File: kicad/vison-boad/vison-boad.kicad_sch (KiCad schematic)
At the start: 29 parts, among them J1 USB_C_Receptacle_USB2.0, J2 Wio Terminal, J3 UART, J4 pin_test, J5 NEO PIXEL, J6 to main, J7 I2C_0, SW1 BOOTSET, SW2 RST, SW3 M1n_RST, U1 RP2040_Stamp, U2 M1n-break, U3 M1n-break, U4 M1n-break, U5 M1n-break, U6 M1n-break

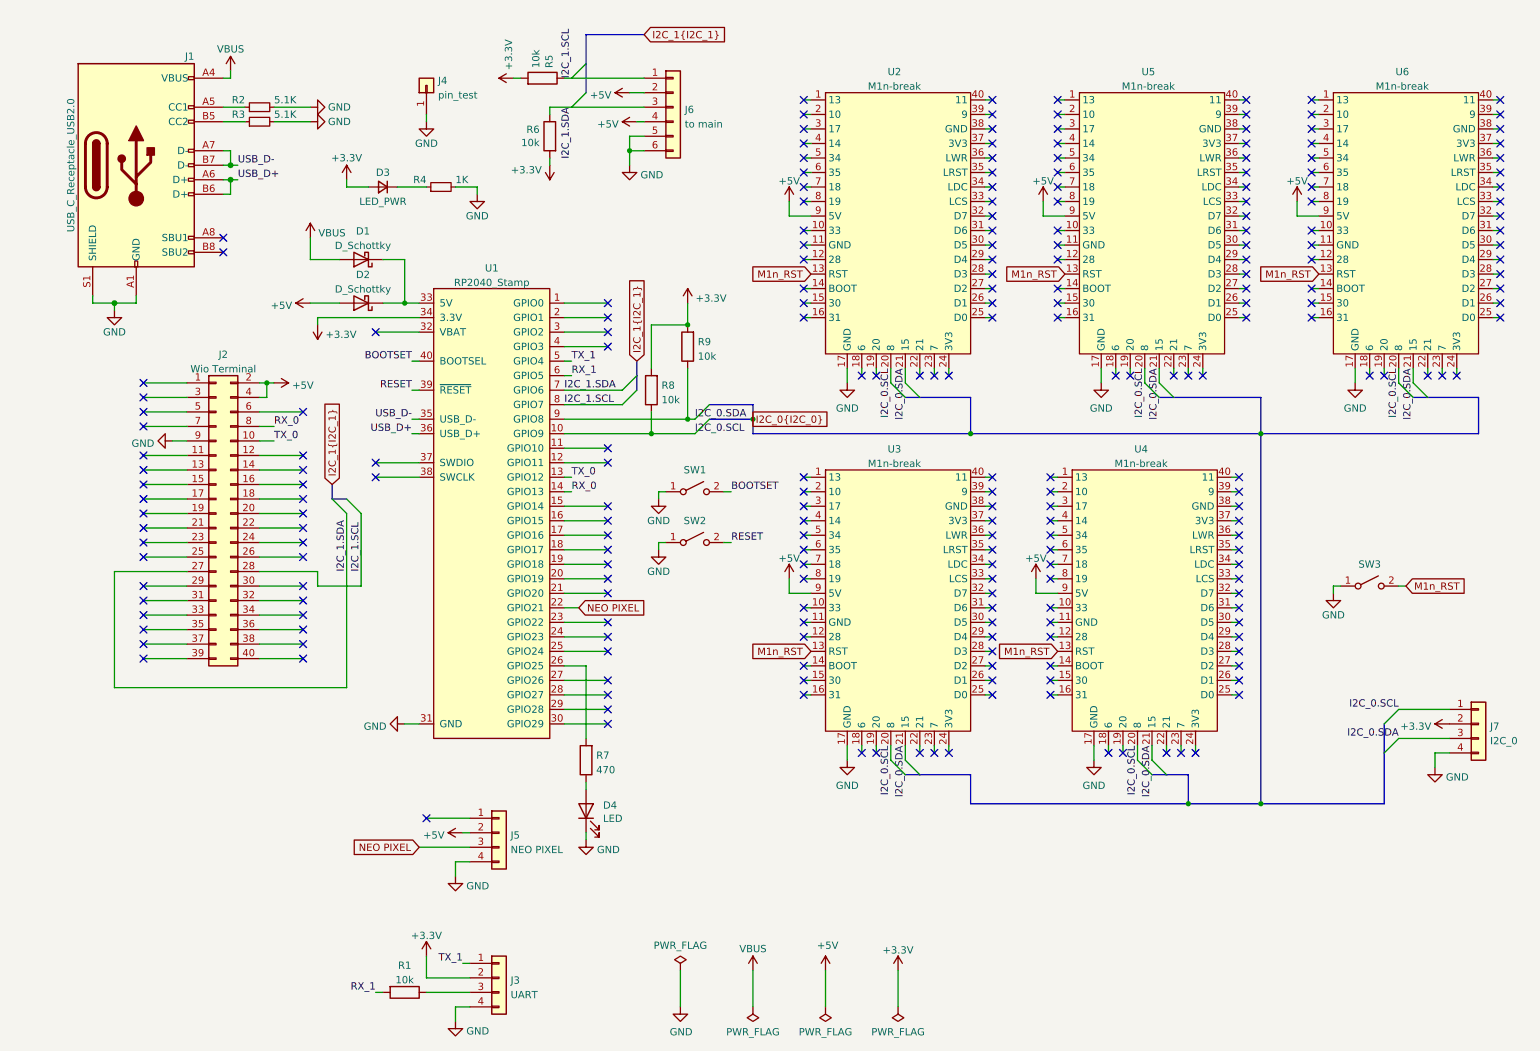
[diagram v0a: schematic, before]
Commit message: bus
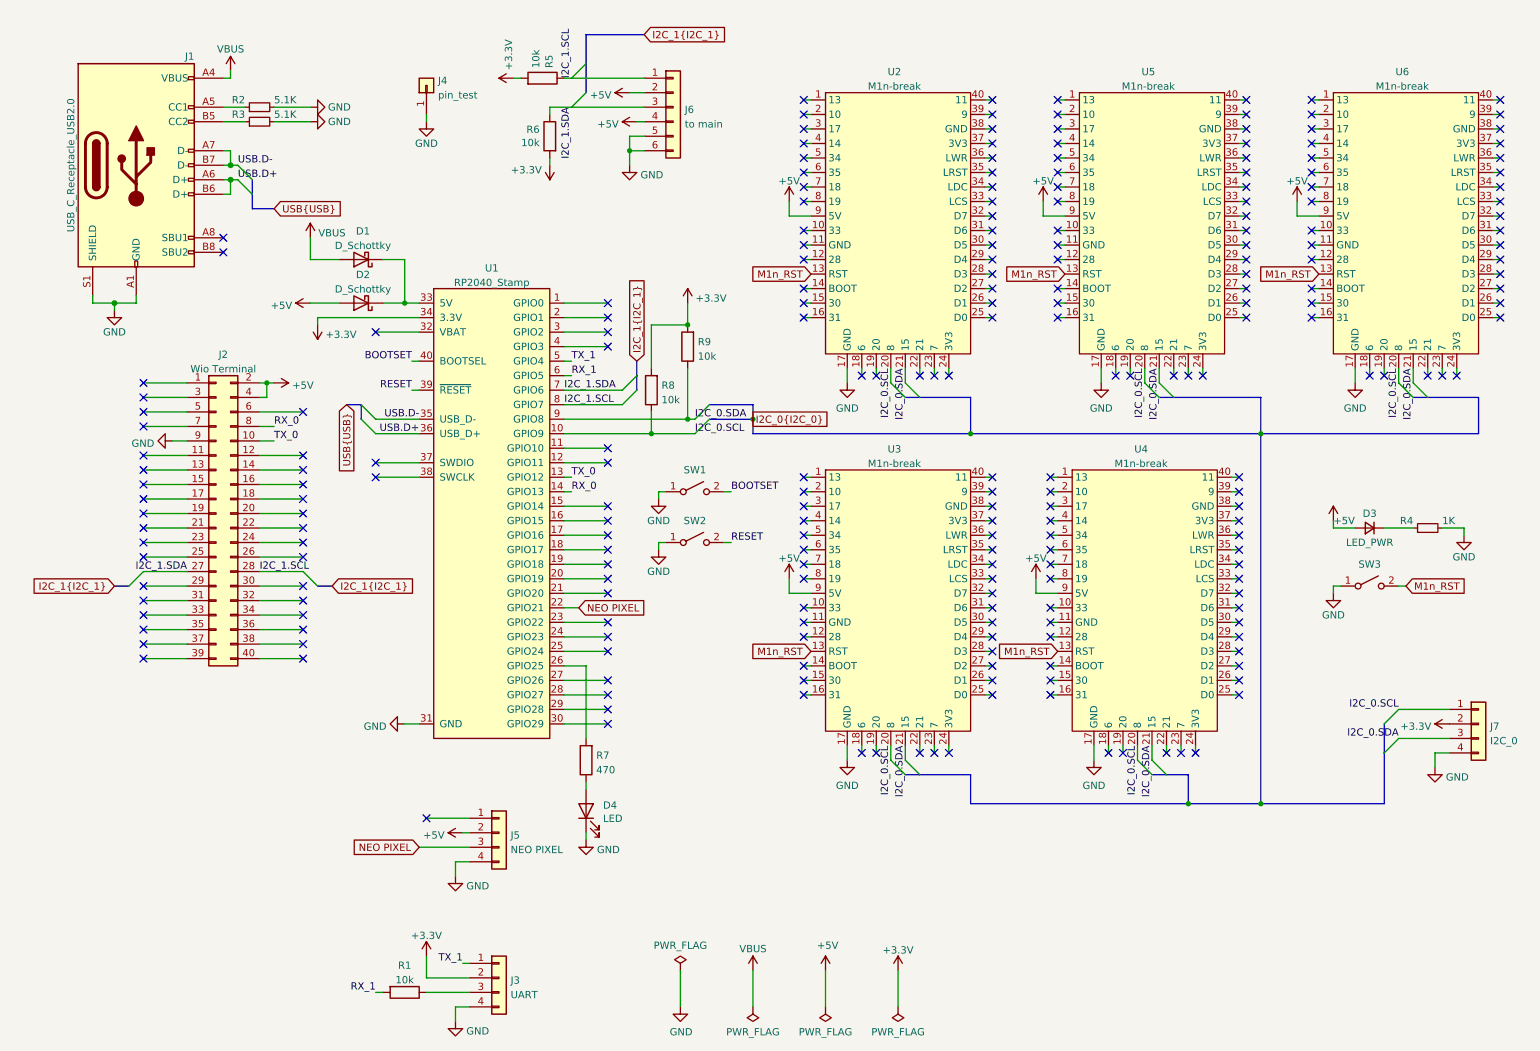
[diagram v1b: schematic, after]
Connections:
- net +3.3V: no longer D3.2 (A)
- net +5V: now also D3.2 (A)
- net USB_D+ renamed USB.D+
- net USB_D- renamed USB.D-
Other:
- moved on the sheet: D3, R4
